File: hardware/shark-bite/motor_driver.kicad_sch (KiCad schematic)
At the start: 59 parts, among them J6 Conn_01x03_Pin, U10 IRFH7440TRPBF, U11 IRFH7440TRPBF, U12 IRFH7440TRPBF, U4 GD32E230G6U6TR, U5 FD6288Q, U6 AOZ1282CI, U7 IRFH7440TRPBF, U8 IRFH7440TRPBF, U9 IRFH7440TRPBF

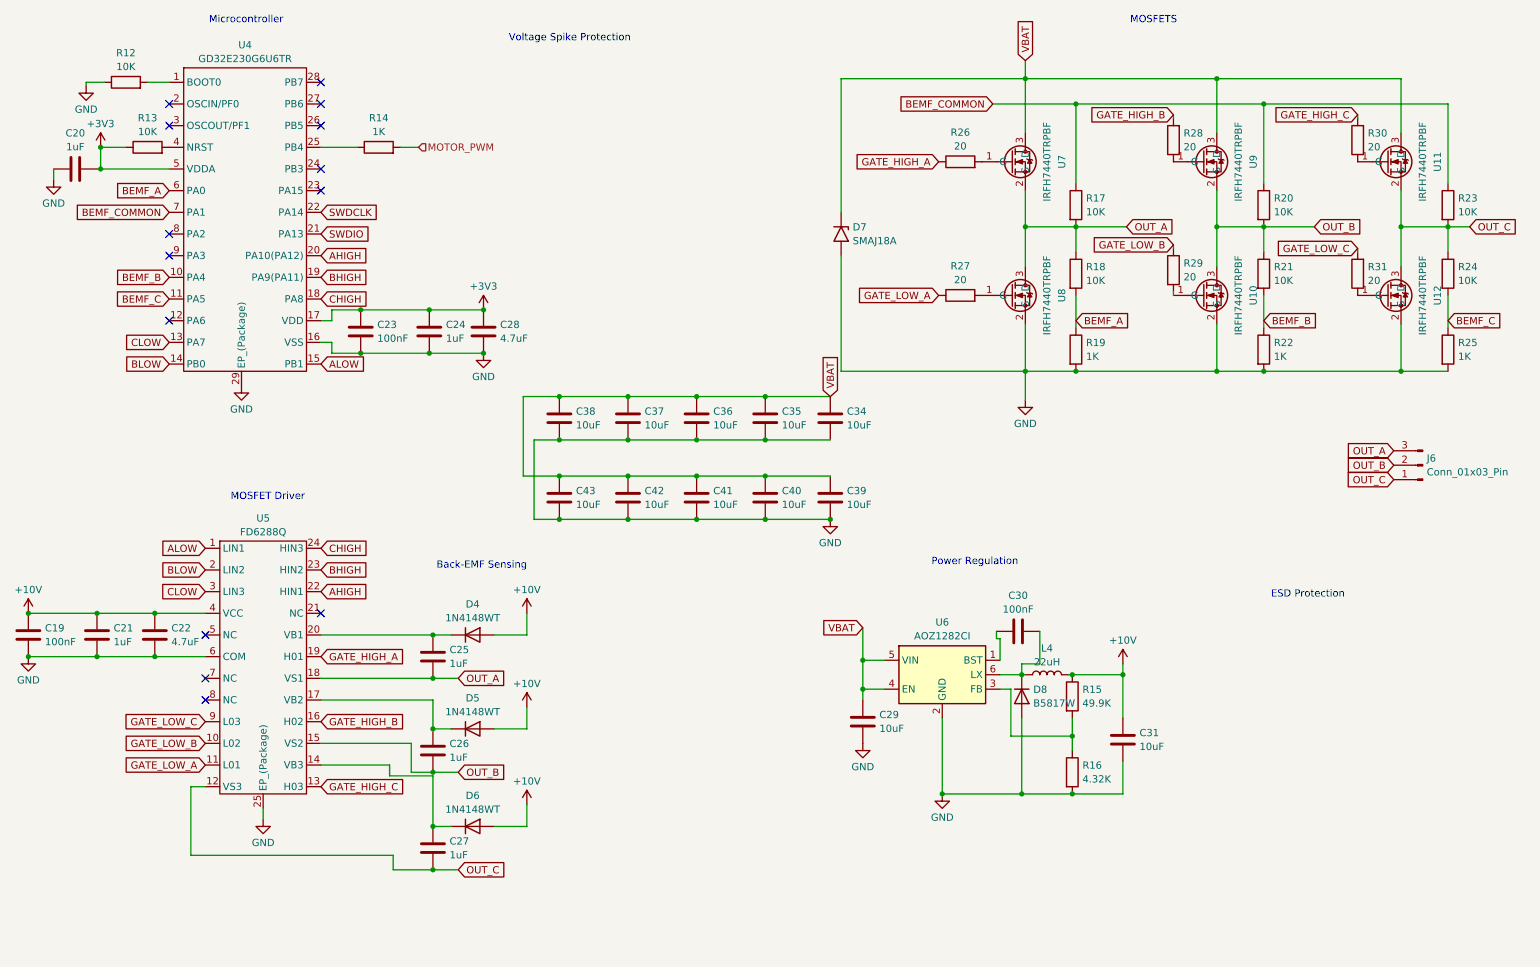
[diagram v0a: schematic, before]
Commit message: V0
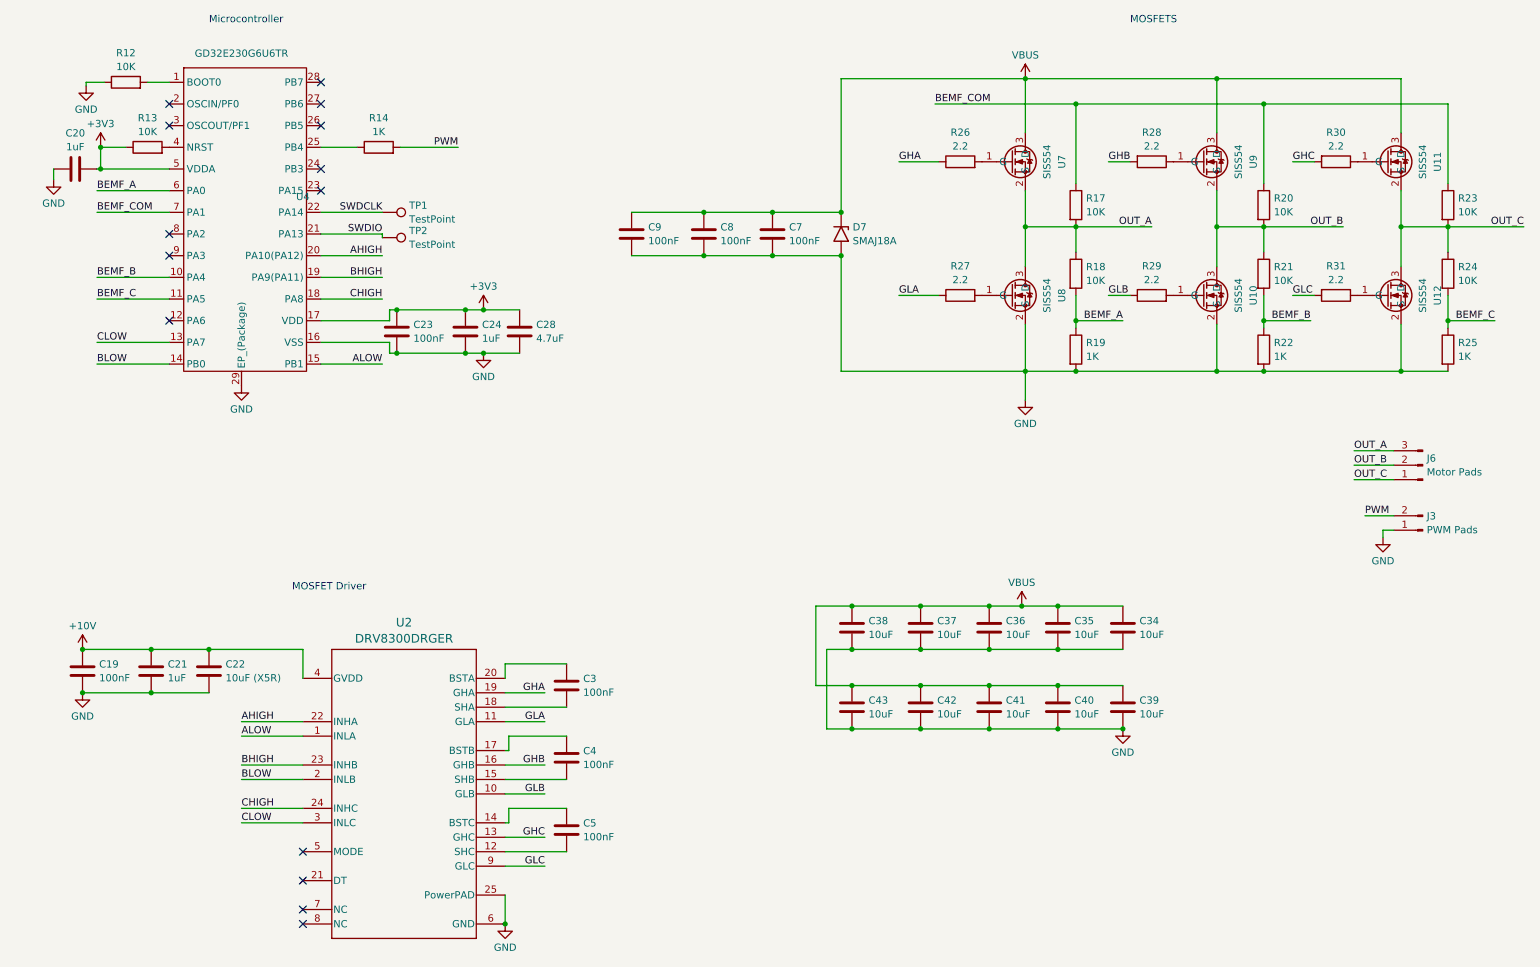
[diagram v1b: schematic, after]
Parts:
- removed C25, C26, C27: 1uF, Capacitor_SMD:C_0402_1005Metric_Pad0.74x0.62mm_HandSolder, symbol Device:C
- removed C29, C31: 10uF, Capacitor_SMD:C_0402_1005Metric_Pad0.74x0.62mm_HandSolder, symbol Device:C
- removed C30: 100nF, Capacitor_SMD:C_0402_1005Metric_Pad0.74x0.62mm_HandSolder, symbol Device:C
- removed D4, D5, D6: 1N4148WT, Diode_SMD:D_SOD-523, symbol Diode:1N4148WT
- removed D8: B5817W, Diode_SMD:D_SOD-123, symbol Device:D
- removed L4: 22uH, Inductor_SMD:L_Bourns_SRP7028A_7.3x6.6mm, symbol Device:L
- removed R15: 49.9K, Resistor_SMD:R_0402_1005Metric, symbol Device:R
- removed R16: 4.32K, Resistor_SMD:R_0402_1005Metric, symbol Device:R
- removed U5: FD6288Q, Package_DFN_QFN:QFN-24-1EP_4x4mm_P0.5mm_EP2.65x2.65mm, symbol Sharkbite:FD6288Q
- removed U6: AOZ1282CI, Package_TO_SOT_SMD:SOT-23-6, symbol Regulator_Switching:AOZ1282CI
- added C3, C4, C5: 100nF, Capacitor_SMD:C_0402_1005Metric_Pad0.74x0.62mm_HandSolder, symbol Device:C
- added C7, C8, C9: 100nF, Capacitor_SMD:C_0603_1608Metric, symbol Device:C
- added J3: PWM Pads, symbol Connector:Conn_01x02_Pin
- added TP1, TP2: TestPoint, symbol Connector:TestPoint
- added U2: DRV8300DRGER, RGE0024B-IPC_A, symbol Sharkbite:DRV8300DRGER
- C22: value 4.7uF -> 10uF (X5R)
- J6: value Conn_01x03_Pin -> Motor Pads
- R26, R27, R28, R29, R30, R31: value 20 -> 2.2
- U10, U11, U12, U7, U8, U9: value IRFH7440TRPBF -> SISS54; footprint Sharkbite:PQFN FET -> Package_DFN_QFN:Infineon_PQFN-22-15-4EP_6x5mm_P0.65mm
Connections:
- net +10V: now also U2.4 (GVDD)
- net AHIGH: now also U2.22 (INHA)
- net ALOW: now also U2.1 (INLA)
- net BHIGH: now also U2.23 (INHB)
- net BLOW: now also U2.2 (INLB)
- net CHIGH: now also U2.24 (INHC)
- net CLOW: now also U2.3 (INLC)
- net GND: now also C7.2, C8.2, C9.2, J3.1 (Pin_1), U2.25 (PowerPAD), U2.6 (GND)
- net SWDCLK: now also TP1.1
- net SWDIO: now also TP2.1
- net BEMF_COMMON renamed BEMF_COM
- net GATE_HIGH_A renamed GHA
- net GHA: now also U2.19 (GHA)
- net GATE_HIGH_B renamed GHB
- net GHB: now also U2.16 (GHB)
- net GATE_HIGH_C renamed GHC
- net GHC: now also U2.13 (GHC)
- net GATE_LOW_A renamed GLA
- net GLA: now also U2.11 (GLA)
- net GATE_LOW_B renamed GLB
- net GLB: now also U2.10 (GLB)
- net GATE_LOW_C renamed GLC
- net GLC: now also U2.9 (GLC)
- net MOTOR_PWM renamed PWM
- net PWM: now also J3.2 (Pin_2)
- net VBAT renamed VBUS
- net VBUS: now also C7.1, C8.1, C9.1
- new net: C5.2, U2.12 (SHC)
- new net: C5.1, U2.14 (BSTC)
- new net: C4.2, U2.15 (SHB)
- new net: C4.1, U2.17 (BSTB)
- new net: C3.2, U2.18 (SHA)
- new net: C3.1, U2.20 (BSTA)
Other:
- note removed: "Back-EMF Sensing"
- note removed: "ESD Protection"
- note removed: "Power Regulation"
- note removed: "Voltage Spike Protection"
- moved on the sheet: C19, C21, C22, C23, C24, C28, C34, C35, C36, C37, C38, C39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
